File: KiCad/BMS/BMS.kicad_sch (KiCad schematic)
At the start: 21 parts, among them J1 PLS-6, J2 BH1,27-10-G, SW1 B3F1060, SW2 MSS-12D16, U1 STM32F405RGTx, Y1 Crystal

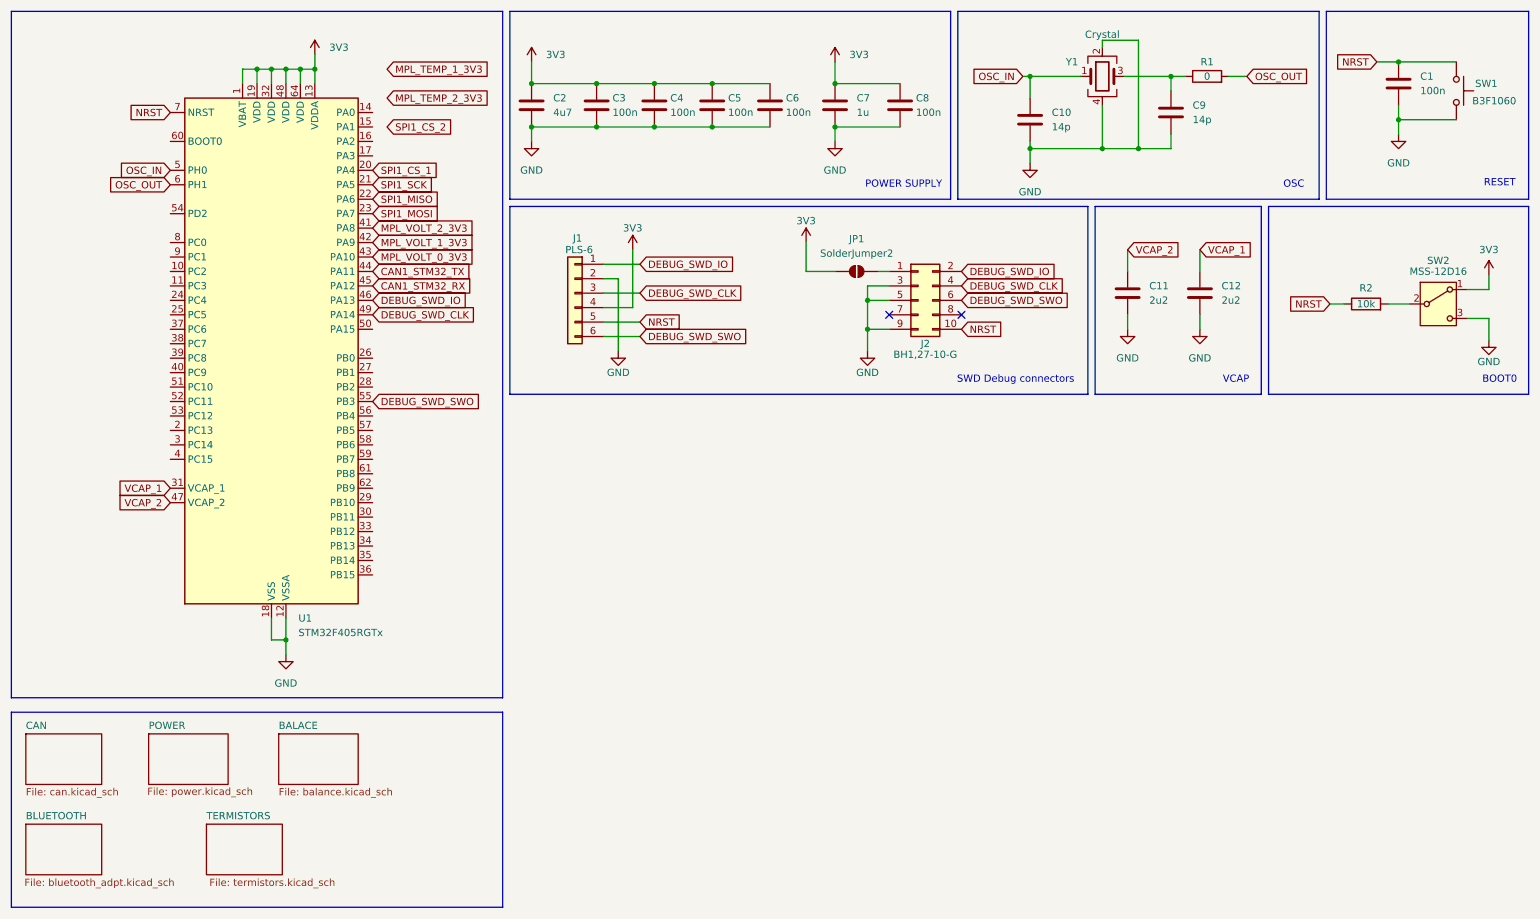
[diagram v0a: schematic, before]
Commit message: 22.03.2025
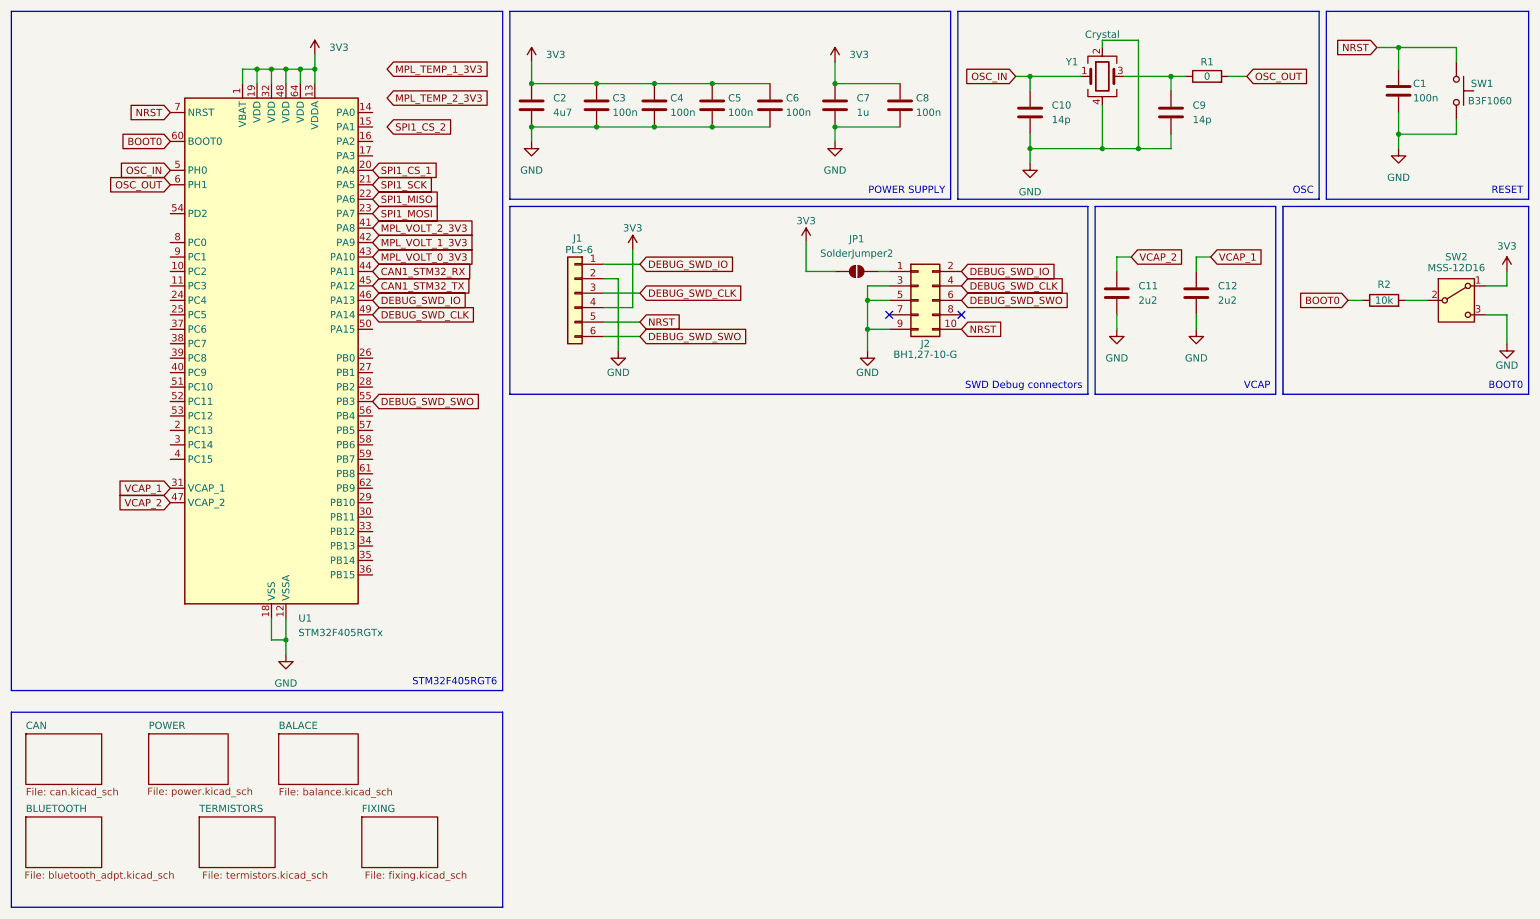
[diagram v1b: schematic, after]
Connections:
- net CAN1_STM32_RX: now also U1.44 (PA11); no longer U1.45 (PA12)
- net CAN1_STM32_TX: now also U1.45 (PA12); no longer U1.44 (PA11)
- net NRST: no longer R2.1
- net BOOT0: now reaches U1.60 (BOOT0)
- net BOOT0: now also R2.1
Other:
- added sheet FIXING (fixing.kicad_sch)
- note removed: "BOOT0"
- note removed: "OSC"
- note removed: "POWER SUPPLY"
- note removed: "RESET"
- note removed: "SWD Debug connectors"
- note removed: "VCAP"
- moved on the sheet: C1, C10, C11, C12, R2, SW2
